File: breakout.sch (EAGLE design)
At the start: 15 parts

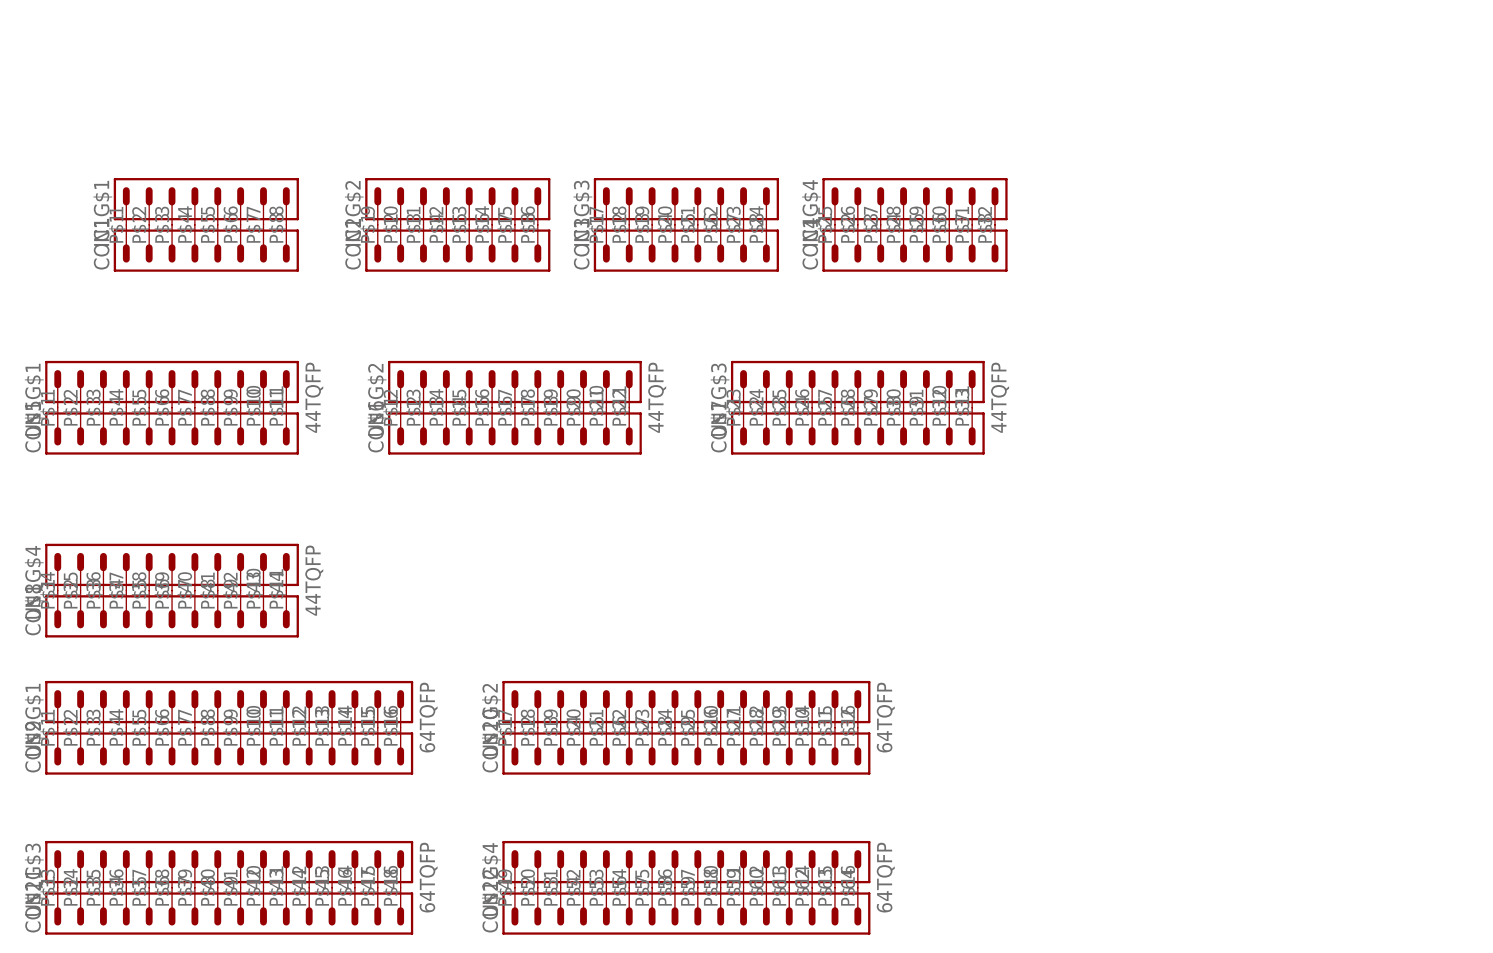
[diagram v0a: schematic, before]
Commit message: Routing and gerbers
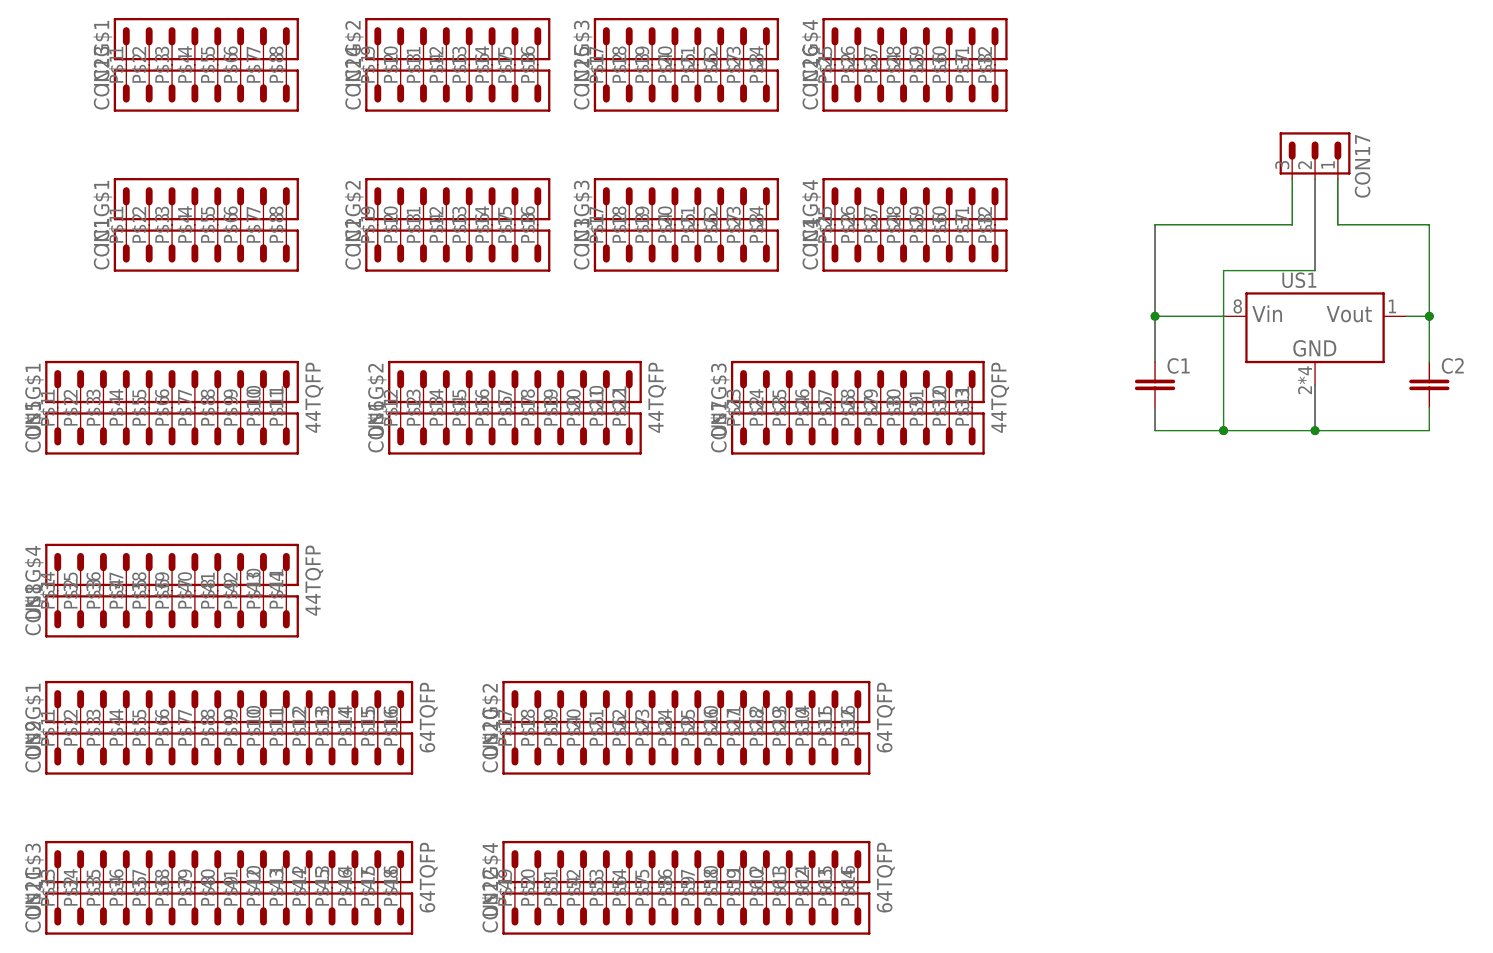
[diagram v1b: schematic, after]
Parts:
- added C1, C2: (no value), PN_default:C0603
- added CON13, CON14, CON15, CON16: (no value), us_obudowy:PIN8X1_SM50
- added CON17: (no value), pins:PIN3X1
- added IC2: (no value), us_obudowy:32MLF
- added US1: (no value), semiconductors:VREG+L-SO8
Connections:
- new net N$141: CON13.1, IC2G$1.1
- new net N$142: CON13.2, IC2G$1.2
- new net N$143: CON13.3, IC2G$1.3
- new net N$144: CON13.4, IC2G$1.4
- new net N$145: CON13.5, IC2G$1.5
- new net N$146: CON13.6, IC2G$1.6
- new net N$147: CON13.7, IC2G$1.7
- new net N$148: CON13.8, IC2G$1.8
- new net N$149: CON14.1, IC2G$2.1
- new net N$150: CON14.2, IC2G$2.2
- new net N$151: CON14.3, IC2G$2.3
- new net N$152: CON14.4, IC2G$2.4
- new net N$153: CON14.5, IC2G$2.5
- new net N$154: CON14.6, IC2G$2.6
- new net N$155: CON14.7, IC2G$2.7
- new net N$156: CON14.8, IC2G$2.8
- new net N$157: CON15.1, IC2G$3.1
- new net N$158: CON15.2, IC2G$3.2
- new net N$159: CON15.3, IC2G$3.3
- new net N$160: CON15.4, IC2G$3.4
- new net N$161: CON15.5, IC2G$3.5
- new net N$162: CON15.6, IC2G$3.6
- new net N$163: CON15.7, IC2G$3.7
- new net N$164: CON15.8, IC2G$3.8
- new net N$165: CON16.1, IC2G$4.1
- new net N$166: CON16.2, IC2G$4.2
- new net N$167: CON16.3, IC2G$4.3
- new net N$168: CON16.4, IC2G$4.4
- new net N$169: CON16.5, IC2G$4.5
- new net N$170: CON16.6, IC2G$4.6
- new net N$171: CON16.7, IC2G$4.7
- new net N$172: CON16.8, IC2G$4.8
- new net N$177: C2.1, CON17.1, US1.OUT
- new net N$178: C1.1, CON17.3, US1.IN
- new net N$179: C1.2, C2.2, CON17.2, US1.GND
